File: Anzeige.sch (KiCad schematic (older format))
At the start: 31 parts, among them J801 Conn_01x04, J802 Conn_01x04, U801 MCP23017_SO

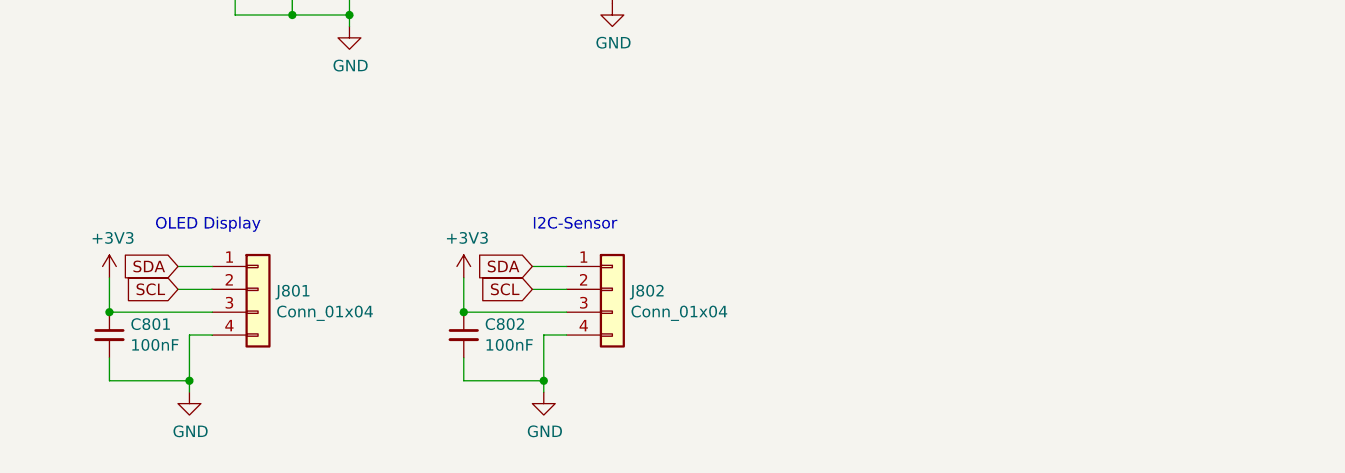
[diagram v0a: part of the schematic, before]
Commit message: fertig zum routen
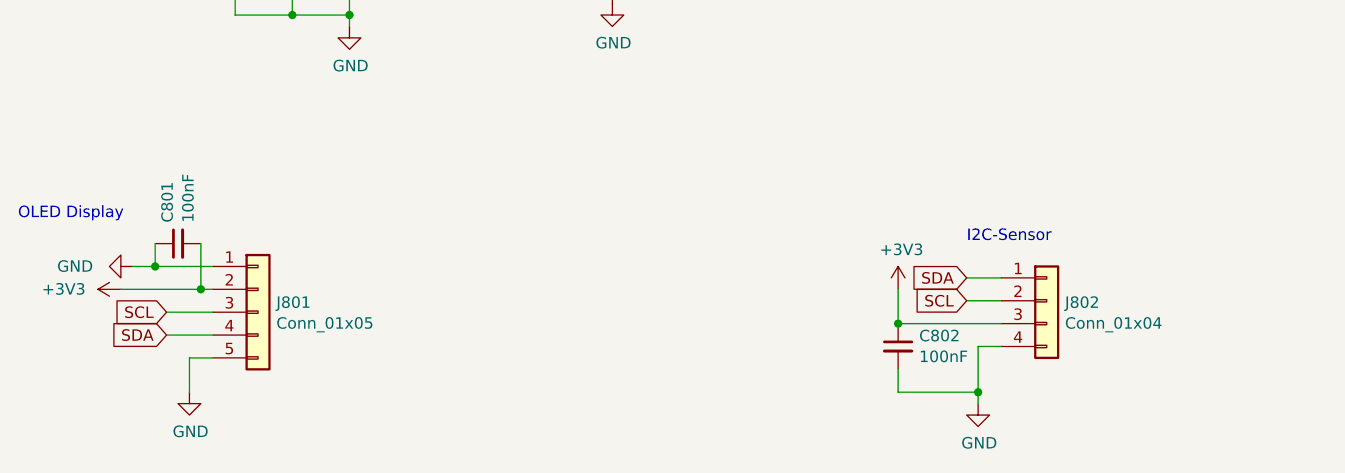
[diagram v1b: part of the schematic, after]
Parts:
- removed J801: Conn_01x04, Connector_PinHeader_2.54mm:PinHeader_1x04_P2.54mm_Vertical, symbol Connector_Generic:Conn_01x04
- added J801: Conn_01x05, Connector:1x04_P2.54mm_1.3OLED, symbol Connector_Generic:Conn_01x05
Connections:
- net +3V3: now also C801.2, J801.2 (Pin_2); no longer C801.1
- net GND: now also C801.1, J801.1 (Pin_1), J801.5 (Pin_5); no longer C801.2
- net SCL: now also J801.3 (Pin_3)
- net SDA: now also J801.4 (Pin_4)
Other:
- moved on the sheet: C801, C802, J802
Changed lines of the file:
@@
 L Connector_Generic:Conn_01x04 J802
 U 1 1 5F610586
-P 3400 4950
-F 0 "J802" H 3480 4942 50  0000 L CNN
-F 1 "Conn_01x04" H 3480 4851 50  0000 L CNN
-F 2 "Connector_PinHeader_2.54mm:PinHeader_1x04_P2.54mm_Vertical" H 3400 4950 50  0001 C CNN
-F 3 "~" H 3400 4950 50  0001 C CNN
-	1    3400 4950
+P 5300 5000
+F 0 "J802" H 5380 4992 50  0000 L CNN
+F 1 "Conn_01x04" H 5380 4901 50  0000 L CNN
+F 2 "Connector_PinHeader_2.54mm:PinHeader_1x04_P2.54mm_Vertical" H 5300 5000 50  0001 C CNN
+F 3 "~" H 5300 5000 50  0001 C CNN
+	1    5300 5000
 	1    0    0    -1
 $EndComp
@@
 L power:GND #PWR0809
 U 1 1 5F61077C
-P 3100 5400
-F 0 "#PWR0809" H 3100 5150 50  0001 C CNN
-F 1 "GND" H 3105 5227 50  0000 C CNN
-F 2 "" H 3100 5400 50  0001 C CNN
-F 3 "" H 3100 5400 50  0001 C CNN
-	1    3100 5400
+P 5000 5450
+F 0 "#PWR0809" H 5000 5200 50  0001 C CNN
+F 1 "GND" H 5005 5277 50  0000 C CNN
+F 2 "" H 5000 5450 50  0001 C CNN
+F 3 "" H 5000 5450 50  0001 C CNN
+	1    5000 5450
 	1    0    0    -1
 $EndComp
 Wire Wire Line
-	3200 5150 3100 5150
+	5100 5200 5000 5200
 Wire Wire Line
-	3100 5150 3100 5350
+	5000 5200 5000 5400
 $Comp
 L power:+3V3 #PWR0807
 U 1 1 5F6121E4
-P 2750 4900
-F 0 "#PWR0807" H 2750 4750 50  0001 C CNN
-F 1 "+3V3" H 2765 5073 50  0000 C CNN
-F 2 "" H 2750 4900 50  0001 C CNN
-F 3 "" H 2750 4900 50  0001 C CNN
-	1    2750 4900
+P 4650 4950
+F 0 "#PWR0807" H 4650 4800 50  0001 C CNN
+F 1 "+3V3" H 4665 5123 50  0000 C CNN
+F 2 "" H 4650 4950 50  0001 C CNN
+F 3 "" H 4650 4950 50  0001 C CNN
+	1    4650 4950
 	1    0    0    -1
 $EndComp
 Wire Wire Line
-	2750 4900 2750 5050
+	4650 4950 4650 5100
 Wire Wire Line
-	2750 5050 3200 5050
+	4650 5100 5100 5100
 $Comp
 L Device:C_Small C802
 U 1 1 5F613EA2
-P 2750 5150
-F 0 "C802" H 2842 5196 50  0000 L CNN
-F 1 "100nF" H 2842 5105 50  0000 L CNN
-F 2 "Capacitor_SMD:C_0603_1608Metric_Pad1.05x0.95mm_HandSolder" H 2750 5150 50  0001 C CNN
-F 3 "~" H 2750 5150 50  0001 C CNN
-	1    2750 5150
+P 4650 5200
+F 0 "C802" H 4742 5246 50  0000 L CNN
+F 1 "100nF" H 4742 5155 50  0000 L CNN
+F 2 "Capacitor_SMD:C_0603_1608Metric_Pad1.05x0.95mm_HandSolder" H 4650 5200 50  0001 C CNN
+F 3 "~" H 4650 5200 50  0001 C CNN
+	1    4650 5200
 	1    0    0    -1
 $EndComp
-Connection ~ 2750 5050
+Connection ~ 4650 5100
 Wire Wire Line
-	2750 5250 2750 5350
+	4650 5300 4650 5400
 Wire Wire Line
-	2750 5350 3100 5350
-Connection ~ 3100 5350
+	4650 5400 5000 5400
+Connection ~ 5000 5400
 Wire Wire Line
-	3100 5350 3100 5400
-Text GLabel 3050 4850 0    50   Input ~ 0
+	5000 5400 5000 5450
+Text GLabel 4950 4900 0    50   Input ~ 0
 SDA
 Wire Wire Line
-	3200 4850 3050 4850
-Text GLabel 3050 4950 0    50   Input ~ 0
+	5100 4900 4950 4900
+Text GLabel 4950 5000 0    50   Input ~ 0
 SCL
 Wire Wire Line
-	3200 4950 3050 4950
-$Comp
-L Connector_Generic:Conn_01x04 J801
-U 1 1 5F61FAF7
-P 1850 4950
-F 0 "J801" H 1930 4942 50  0000 L CNN
-F 1 "Conn_01x04" H 1930 4851 50  0000 L CNN
-F 2 "Connector_PinHeader_2.54mm:PinHeader_1x04_P2.54mm_Vertical" H 1850 4950 50  0001 C CNN
-F 3 "~" H 1850 4950 50  0001 C CNN
-	1    1850 4950
-	1    0    0    -1
-$EndComp
+	5100 5000 4950 5000
 $Comp
 L power:GND #PWR0802
@@
 	1    0    0    -1
 $EndComp
-Wire Wire Line
-	1650 5150 1550 5150
-Wire Wire Line
-	1550 5150 1550 5350
 $Comp
 L power:+3V3 #PWR0801
 U 1 1 5F61FB06
-P 1200 4900
-F 0 "#PWR0801" H 1200 4750 50  0001 C CNN
-F 1 "+3V3" H 1215 5073 50  0000 C CNN
-F 2 "" H 1200 4900 50  0001 C CNN
-F 3 "" H 1200 4900 50  0001 C CNN
-	1    1200 4900
+P 1250 4950
+F 0 "#PWR0801" H 1250 4800 50  0001 C CNN
+F 1 "+3V3" V 1250 5200 50  0000 C CNN
+F 2 "" H 1250 4950 50  0001 C CNN
+F 3 "" H 1250 4950 50  0001 C CNN
+	1    1250 4950
+	0    -1   -1   0
+$EndComp
+$Comp
+L Device:C_Small C801
+U 1 1 5F61FB0E
+P 1500 4750
+F 0 "C801" H 1592 4796 50  0000 L CNN
+F 1 "100nF" H 1592 4705 50  0000 L CNN
+F 2 "Capacitor_SMD:C_0603_1608Metric_Pad1.05x0.95mm_HandSolder" H 1500 4750 50  0001 C CNN
+F 3 "~" H 1500 4750 50  0001 C CNN
+	1    1500 4750
+	0    -1   -1   0
+$EndComp
+Text GLabel 1450 5150 0    50   Input ~ 0
+SDA
+Wire Wire Line
+	1650 4850 1400 4850
+Text GLabel 1450 5050 0    50   Input ~ 0
+SCL
+Wire Wire Line
+	1650 4950 1600 4950
+Text Notes 800  4650 0    50   ~ 0
+OLED Display
+Text Notes 4950 4750 0    50   ~ 0
+I2C-Sensor
+$Comp
+L Connector_Generic:Conn_01x05 J801
+U 1 1 5E98BB32
+P 1850 5050
+F 0 "J801" H 1930 5092 50  0000 L CNN
+F 1 "Conn_01x05" H 1930 5001 50  0000 L CNN
+F 2 "Connector:1x04_P2.54mm_1.3OLED" H 1850 5050 50  0001 C CNN
+F 3 "~" H 1850 5050 50  0001 C CNN
+	1    1850 5050
 	1    0    0    -1
 $EndComp
 Wire Wire Line
-	1200 4900 1200 5050
+	1650 5250 1550 5250
 Wire Wire Line
-	1200 5050 1650 5050
+	1550 5250 1550 5400
 $Comp
-L Device:C_Small C801
-U 1 1 5F61FB0E
-P 1200 5150
-F 0 "C801" H 1292 5196 50  0000 L CNN
-F 1 "100nF" H 1292 5105 50  0000 L CNN
-F 2 "Capacitor_SMD:C_0603_1608Metric_Pad1.05x0.95mm_HandSolder" H 1200 5150 50  0001 C CNN
-F 3 "~" H 1200 5150 50  0001 C CNN
-	1    1200 5150
-	1    0    0    -1
+L power:GND #PWR0192
+U 1 1 5E99C353
+P 1300 4850
+F 0 "#PWR0192" H 1300 4600 50  0001 C CNN
+F 1 "GND" V 1300 4600 50  0000 C CNN
+F 2 "" H 1300 4850 50  0001 C CNN
+F 3 "" H 1300 4850 50  0001 C CNN
+	1    1300 4850
+	0    1    1    0
 $EndComp
-Connection ~ 1200 5050
 Wire Wire Line
-	1200 5250 1200 5350
+	1650 5150 1450 5150
 Wire Wire Line
-	1200 5350 1550 5350
-Connection ~ 1550 5350
+	1650 5050 1450 5050
 Wire Wire Line
-	1550 5350 1550 5400
-Text GLabel 1500 4850 0    50   Input ~ 0
-SDA
+	1400 4750 1400 4850
+Connection ~ 1400 4850
 Wire Wire Line
-	1650 4850 1500 4850
-Text GLabel 1500 4950 0    50   Input ~ 0
-SCL
+	1400 4850 1300 4850
 Wire Wire Line
-	1650 4950 1500 4950
-Text Notes 1400 4700 0    50   ~ 0
-OLED Display
-Text Notes 3050 4700 0    50   ~ 0
-I2C-Sensor
+	1600 4750 1600 4950
+Connection ~ 1600 4950
+Wire Wire Line
+	1600 4950 1250 4950
 $EndSCHEMATC
